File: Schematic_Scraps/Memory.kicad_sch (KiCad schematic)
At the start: 4 parts, among them U10 КС573РФ2/2716 (N1), U11 КС573РФ2/2716 (N2), U12 КС573РФ2/2716 (N3), U4 К555ТЛ2 (74LS138)

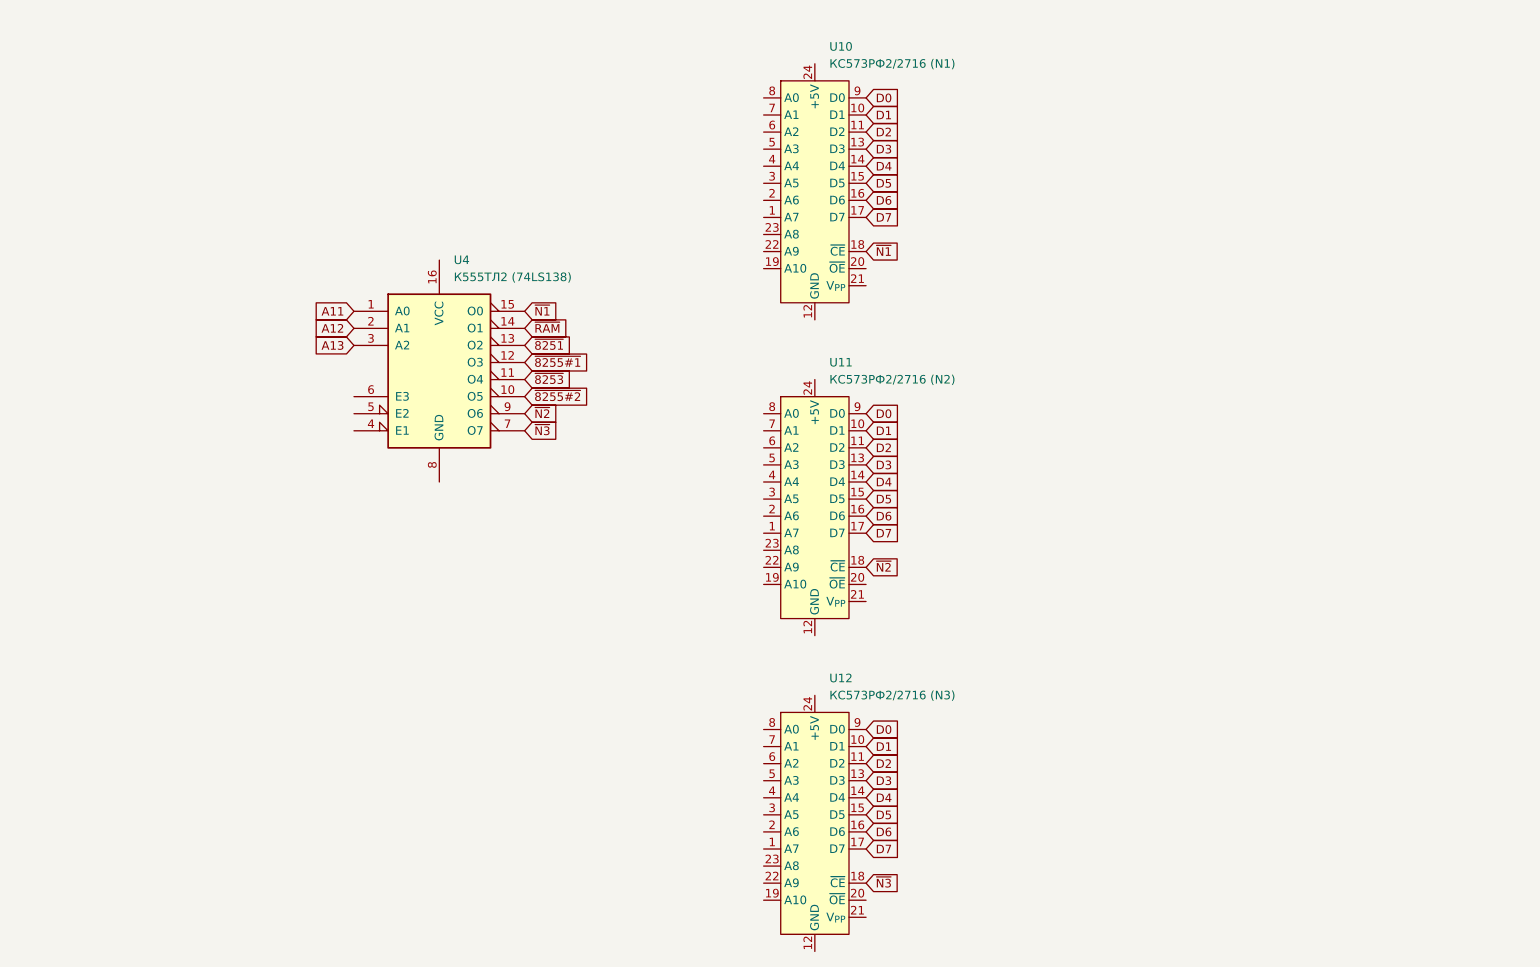
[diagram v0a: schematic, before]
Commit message: Analysis progress
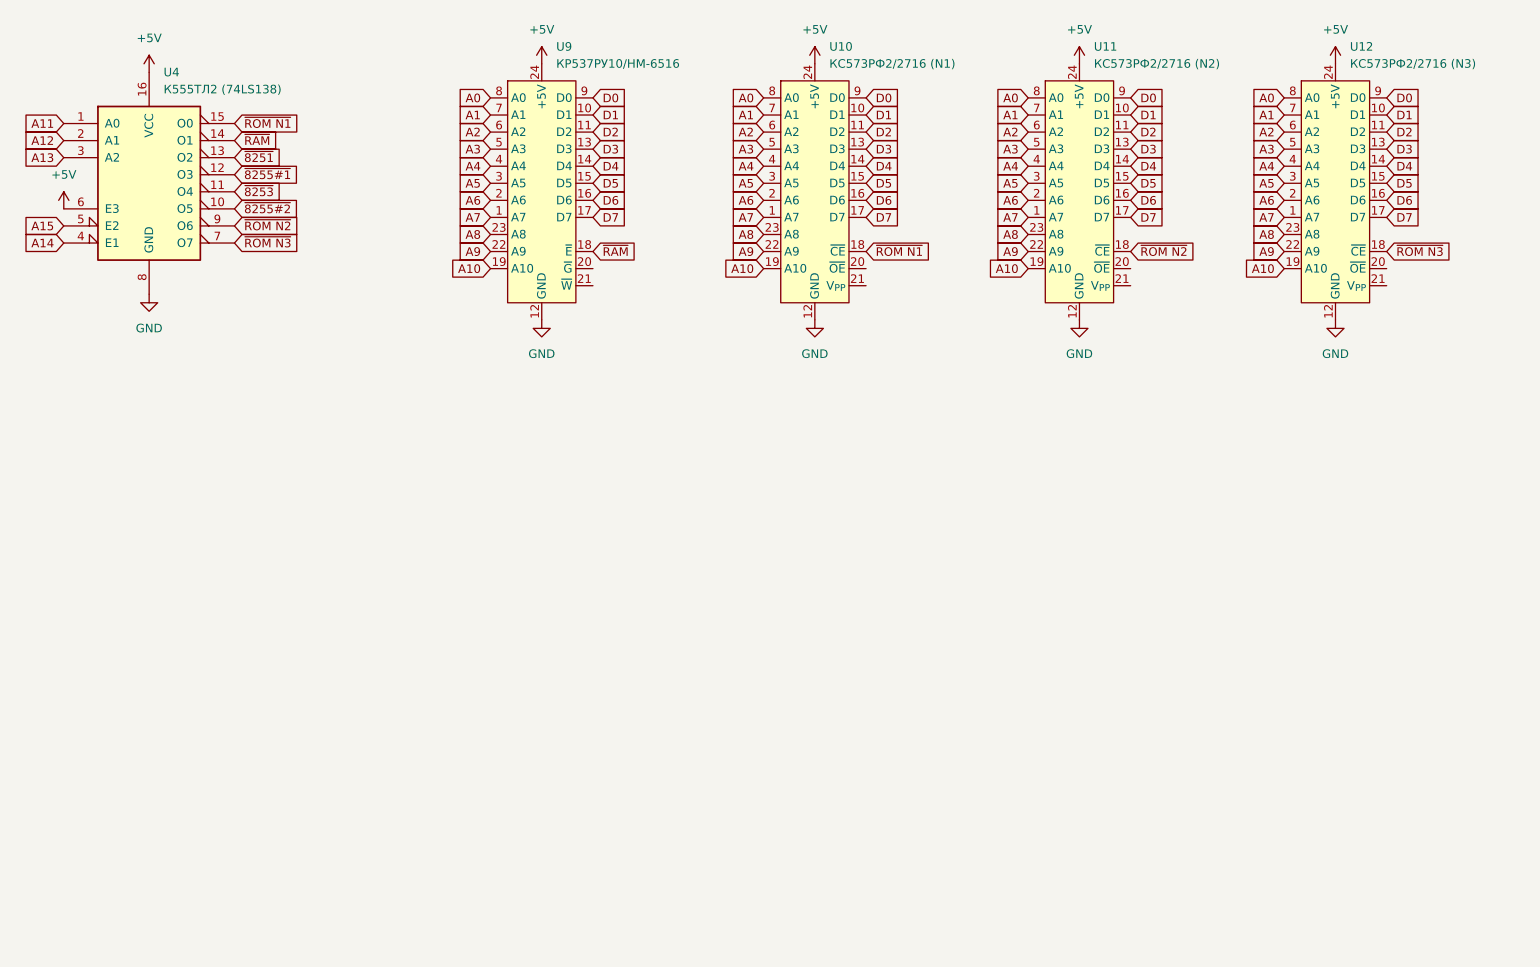
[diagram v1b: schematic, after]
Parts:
- added U9: КР537РУ10/HM-6516, Package_DIP:DIP-24_W15.24mm, symbol Clueless_Engineer:HM-6516
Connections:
- net D0: now also U9.9 (D0)
- net D1: now also U9.10 (D1)
- net D2: now also U9.11 (D2)
- net D3: now also U9.13 (D3)
- net D4: now also U9.14 (D4)
- net D5: now also U9.15 (D5)
- net D6: now also U9.16 (D6)
- net D7: now also U9.17 (D7)
- net ~{RAM}: now also U9.18 (~{E})
- net A7: now reaches U10.1 (A7)
- net A7: now also U11.1 (A7), U12.1 (A7), U9.1 (A7)
- net GND: now reaches U10.12 (GND)
- net GND: now also U11.12 (GND), U12.12 (GND), U4.8 (GND), U9.12 (GND)
- net A10: now reaches U10.19 (A10)
- net A10: now also U11.19 (A10), U12.19 (A10), U9.19 (A10)
- net A6: now reaches U10.2 (A6)
- net A6: now also U11.2 (A6), U12.2 (A6), U9.2 (A6)
- net A9: now reaches U10.22 (A9)
- net A9: now also U11.22 (A9), U12.22 (A9), U9.22 (A9)
- net A8: now reaches U10.23 (A8)
- net A8: now also U11.23 (A8), U12.23 (A8), U9.23 (A8)
- net +5V: now reaches U10.24 (+5V)
- net +5V: now also U11.24 (+5V), U12.24 (+5V), U4.16 (VCC), U4.6 (E3), U9.24 (+5V)
- net A5: now reaches U10.3 (A5)
- net A5: now also U11.3 (A5), U12.3 (A5), U9.3 (A5)
- net A4: now reaches U10.4 (A4)
- net A4: now also U11.4 (A4), U12.4 (A4), U9.4 (A4)
- net A3: now reaches U10.5 (A3)
- net A3: now also U11.5 (A3), U12.5 (A3), U9.5 (A3)
- net A2: now reaches U10.6 (A2)
- net A2: now also U11.6 (A2), U12.6 (A2), U9.6 (A2)
- net A1: now reaches U10.7 (A1)
- net A1: now also U11.7 (A1), U12.7 (A1), U9.7 (A1)
- net A0: now reaches U10.8 (A0)
- net A0: now also U11.8 (A0), U12.8 (A0), U9.8 (A0)
- net A14: now reaches U4.4 (E1)
- net A15: now reaches U4.5 (E2)
- net ~{N1} renamed ~{ROM N1}
- net ~{N2} renamed ~{ROM N2}
- net ~{N3} renamed ~{ROM N3}
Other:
- moved on the sheet: U11, U12, U4

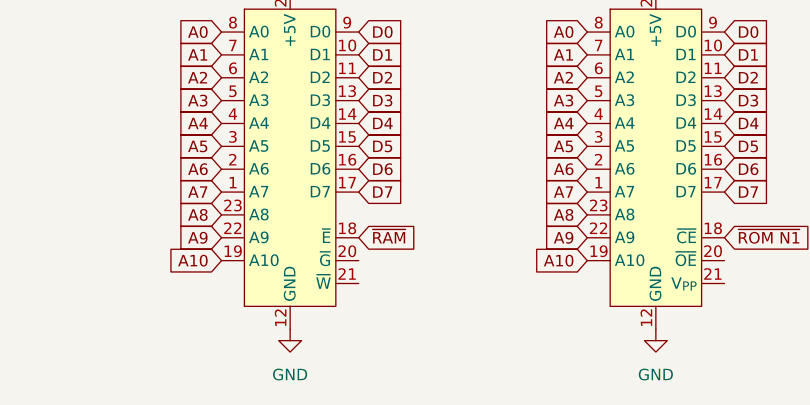
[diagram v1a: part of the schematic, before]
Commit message: Reverse engineering progress
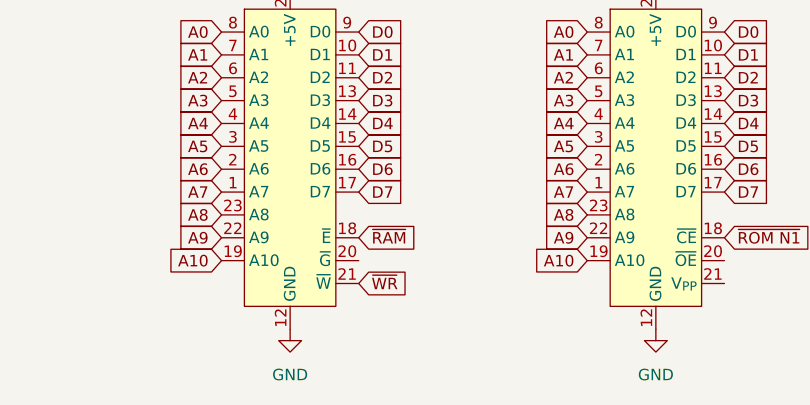
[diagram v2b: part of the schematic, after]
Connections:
- net ~{WR}: now reaches U9.21 (~{W})
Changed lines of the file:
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@@
+		)
+	)
+	(global_label "~{WR}"
+		(shape input)
+		(at 113.03 58.42 0)
+		(fields_autoplaced yes)
+		(effects
+			(font
+				(size 1.27 1.27)
+			)
+			(justify left)
+		)
+		(property "Intersheetrefs" "${INTERSHEET_REFS}"
+			(at 118.7366 58.42 0)
+			(effects
+				(font
+					(size 1.27 1.27)
+				)
+				(justify left)
+				(hide yes)
+			)
 		)
 	)

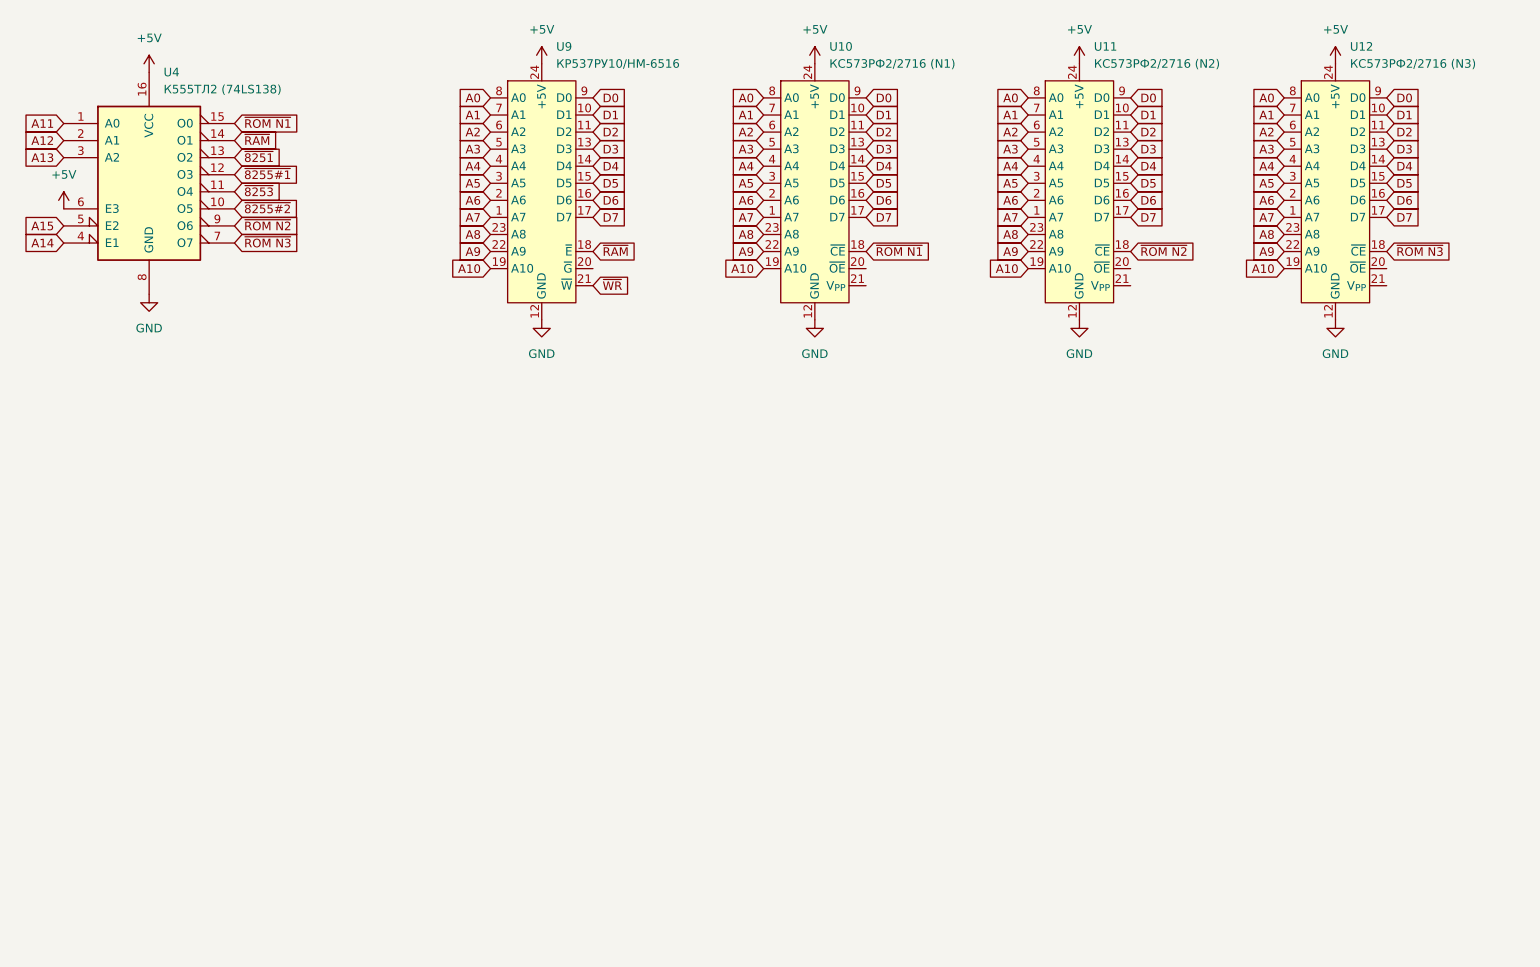
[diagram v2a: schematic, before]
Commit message: Further reverse engineering progress
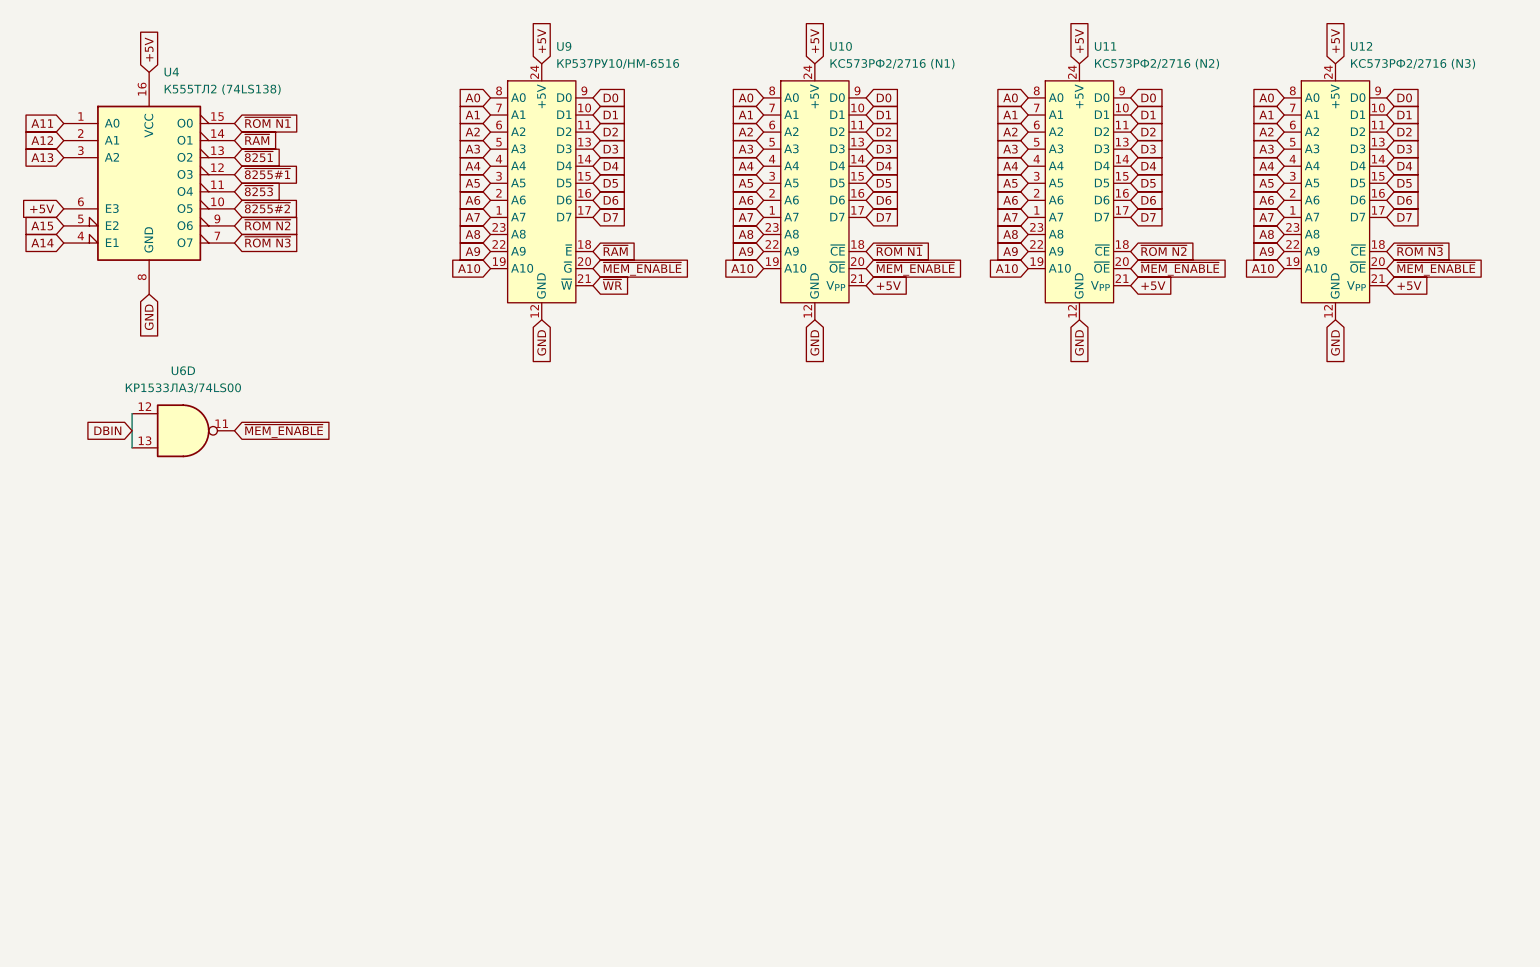
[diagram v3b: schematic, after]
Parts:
- added U6: КР1533ЛА3/74LS00, symbol 74xx:74LS00
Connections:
- net +5V: now also U10.21 (V_{PP}), U11.21 (V_{PP}), U12.21 (V_{PP})
- net ~{MEM_ENABLE}: now reaches U10.20 (~{OE})
- net ~{MEM_ENABLE}: now also U11.20 (~{OE}), U12.20 (~{OE}), U9.20 (~{G}), U6.11
- new net DBIN: U6.12, U6.13
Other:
- company: (none) -> Brett Hallen
- title: (none) -> Rhythm Keyboard (Ритм Клав)

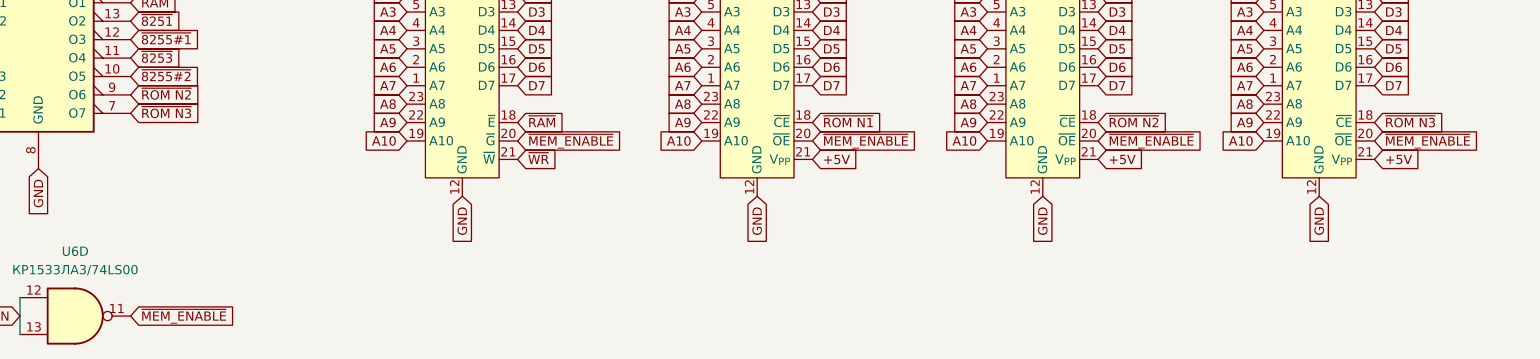
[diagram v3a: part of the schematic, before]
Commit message: 19-May reverse engineering progress
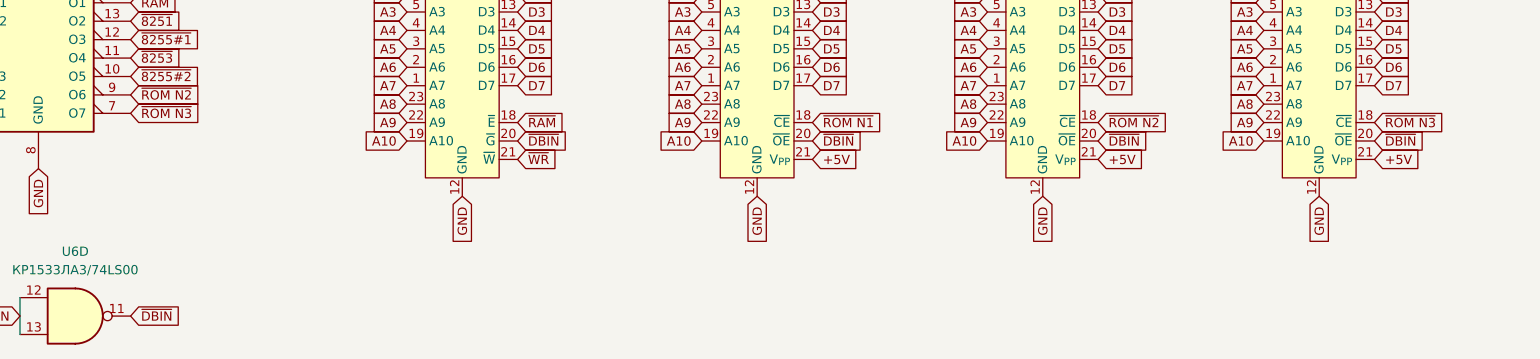
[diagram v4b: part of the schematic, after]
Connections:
- net ~{MEM_ENABLE} renamed ~{DBIN}
